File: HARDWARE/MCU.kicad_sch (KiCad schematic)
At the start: 1 part, among them U2 STM32H750VBTx

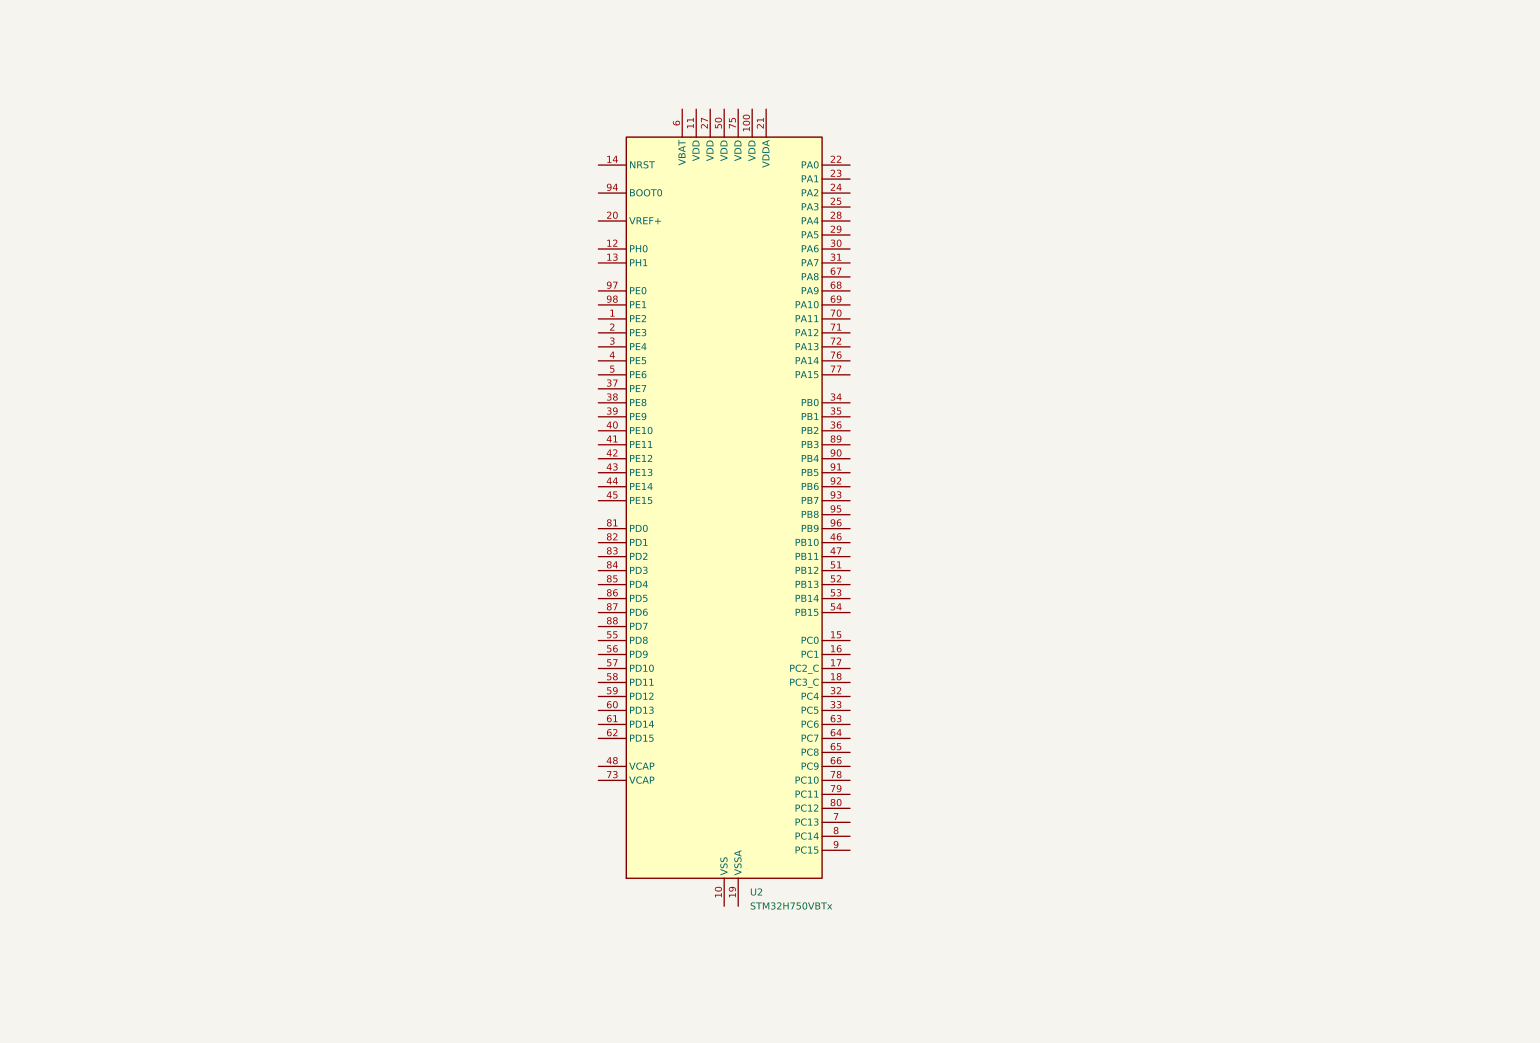
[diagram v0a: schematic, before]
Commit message: Update first version of schematic
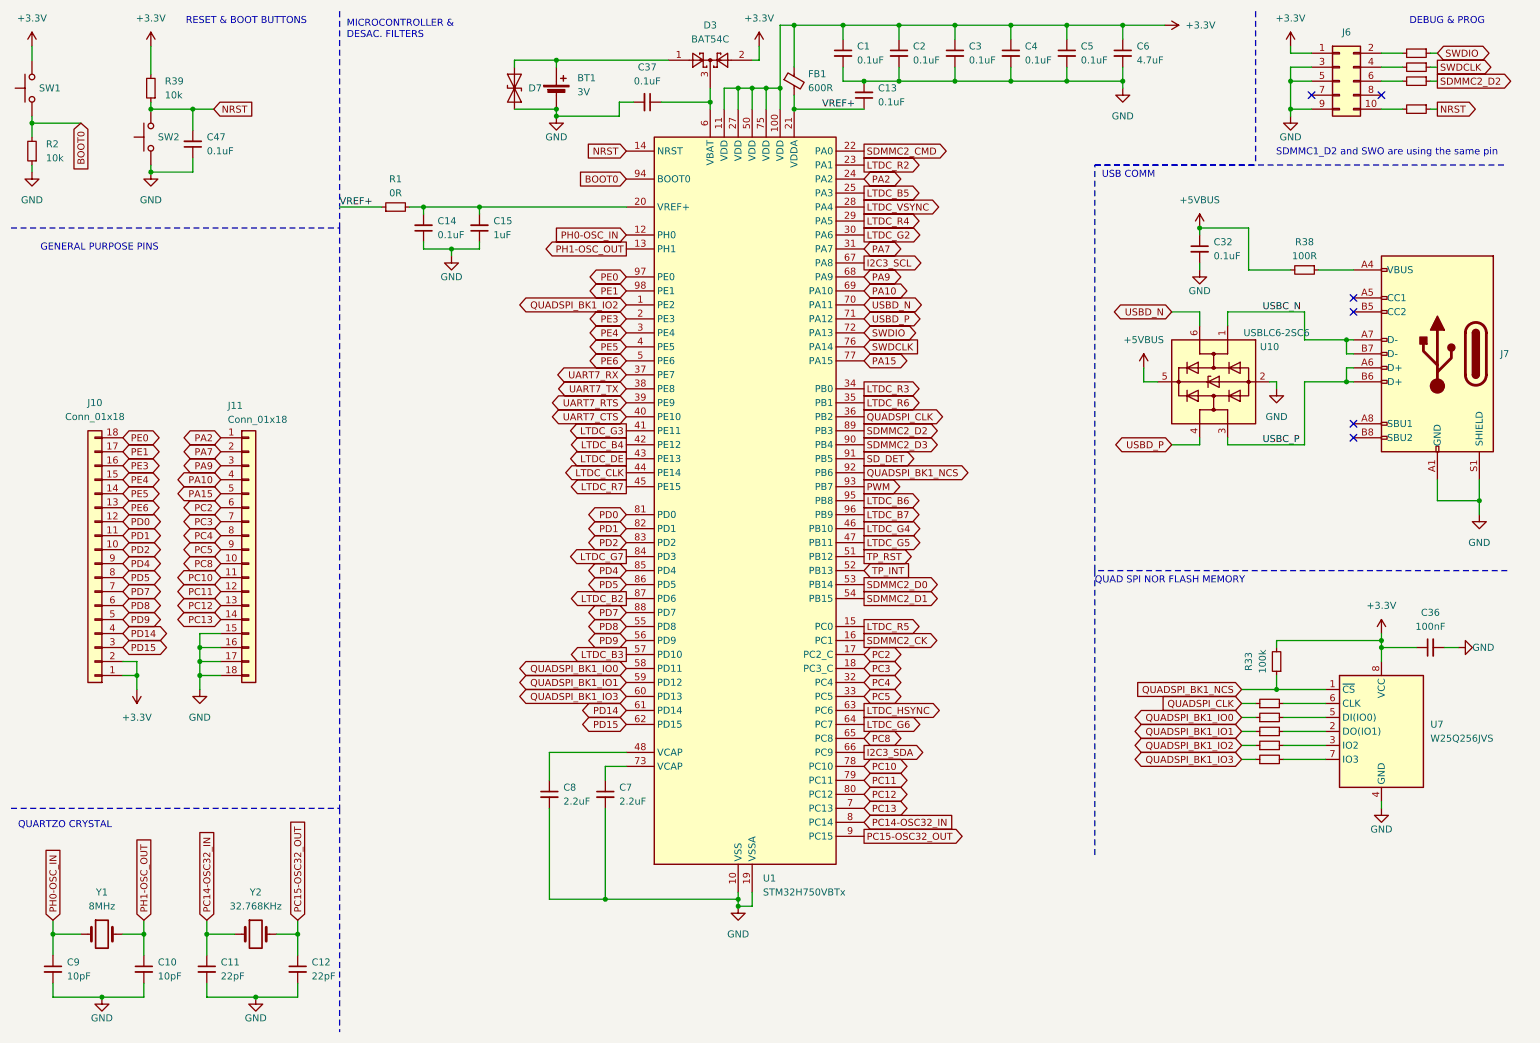
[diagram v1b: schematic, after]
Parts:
- removed U2: STM32H750VBTx, Package_QFP:LQFP-100_14x14mm_P0.5mm, symbol MCU_ST_STM32H7:STM32H750VBTx
- added BT1: 3V, BS-12-B-___002:BS-12-B-1A, symbol Device:Battery_Cell
- added C1, C13, C14, C2, C3, C32, C37, C4, C47, C5: 0.1uF, Capacitor_SMD:C_0603_1608Metric, symbol Device:C_Small
- added C10, C9: 10pF, Capacitor_SMD:C_0603_1608Metric, symbol Device:C_Small
- added C11, C12: 22pF, Capacitor_SMD:C_0603_1608Metric, symbol Device:C_Small
- added C15: 1uF, Capacitor_SMD:C_0603_1608Metric, symbol Device:C_Small
- added C36: 100nF, Capacitor_SMD:C_0603_1608Metric, symbol Device:C_Small
- added C6: 4.7uF, Capacitor_SMD:C_0603_1608Metric, symbol Device:C_Small
- added C7, C8: 2.2uF, Capacitor_SMD:C_0603_1608Metric, symbol Device:C_Small
- added D3: BAT54C, Package_TO_SOT_SMD:SOT-23, symbol Diode:BAT54C
- added D7: ESD9B3.3ST5G, Diode_SMD:D_SOD-923, symbol Diode:ESD9B3.3ST5G
- added FB1: 600R, Inductor_SMD:L_0603_1608Metric, symbol Device:FerriteBead_Small
- added J10, J11: Conn_01x18, Connector_JST:JST_XA_B18B-XASK-1_1x18_P2.50mm_Vertical, symbol Connector_Generic:Conn_01x18
- added J6: Conn_02x05_Odd_Even, Connector_PinHeader_1.27mm:PinHeader_2x05_P1.27mm_Vertical_SMD, symbol Connector_Generic:Conn_02x05_Odd_Even
- added J7: USB_C_Receptacle_USB2.0, Connector_USB:USB_C_Receptacle_G-Switch_GT-USB-7010ASV, symbol Connector:USB_C_Receptacle_USB2.0
- added R1: 0R, Resistor_SMD:R_0603_1608Metric, symbol Device:R_Small
- added R2, R39: 10k, Resistor_SMD:R_0603_1608Metric, symbol Device:R_Small
- added R28, R29, R30, R31, R32: 33R, Resistor_SMD:R_0603_1608Metric, symbol Device:R_Small
- added R33: 100k, Resistor_SMD:R_0603_1608Metric, symbol Device:R_Small
- added R34, R35, R36, R37: 22R, Resistor_SMD:R_0603_1608Metric, symbol Device:R_Small
- added R38: 100R, Resistor_SMD:R_0603_1608Metric, symbol Device:R_Small
- added SW1, SW2: SW_Push, Button_Switch_SMD:SW_SPST_CK_RS282G05A3, symbol Switch:SW_Push
- added U1: STM32H750VBTx, Package_QFP:LQFP-100_14x14mm_P0.5mm, symbol MCU_ST_STM32H7:STM32H750VBTx
- added U10: USBLC6-2SC6, Package_TO_SOT_SMD:SOT-23-6, symbol Power_Protection:USBLC6-2SC6
- added U7: W25Q256JVS, Package_SON:WSON-8-1EP_8x6mm_P1.27mm_EP3.4x4.3mm, symbol Memory_Flash:W25Q128JVS
- added Y1: 8MHz, Crystal:Crystal_SMD_Abracon_ABM3-2Pin_5.0x3.2mm, symbol Device:Crystal
- added Y2: 32.768KHz, Crystal:Crystal_SMD_3215-2Pin_3.2x1.5mm, symbol Device:Crystal
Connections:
- new net: R32.2, U7.6 (CLK)
- new net: J6.10 (Pin_10), R37.2
- new net: BT1.1 (+), D3.1, D7.2 (A2)
- new net: R31.2, U7.7 (IO3)
- new net: R29.2, U7.2 (DO(IO1))
- new net: R30.2, U7.3 (IO2)
- new net: R28.2, U7.5 (DI(IO0))
- new net: J6.2 (Pin_2), R34.2
- new net: C7.1, U1.73 (VCAP)
- new net: C14.2, C15.2, R1.2, U1.20 (VREF+)
- new net: J7.A4 (VBUS), J7.A9 (VBUS), J7.B4 (VBUS), J7.B9 (VBUS), R38.1
- new net: J6.4 (Pin_4), R35.2
- new net: J6.6 (Pin_6), R36.2
- new net: C8.1, U1.48 (VCAP)
- new net: C37.1, D3.3, U1.6 (VBAT)
- new net +3.3V: C1.1, C2.1, C3.1, C36.1, C4.1, C5.1, C6.1, D3.2, FB1.1, J10.1 (Pin_1), J10.2 (Pin_2), J6.1 (Pin_1), R33.2, R39.2, SW1.2, U1.100 (VDD), U1.11 (VDD), U1.27 (VDD), U1.50 (VDD), U1.75 (VDD), U7.8 (VCC)
- new net +5VBUS: C32.1, R38.2, U10.5 (VBUS)
- new net BOOT0: R2.2, SW1.1, U1.94 (BOOT0)
- new net GND: BT1.2 (-), C1.2, C10.2, C11.2, C12.2, C13.2, C14.1, C15.1, C2.2, C3.2, C32.2, C36.2, C37.2, C4.2, C47.1, C5.2, C6.2, C7.2, C8.2, C9.2, D7.1 (A1), J11.15 (Pin_15), J11.16 (Pin_16), J11.17 (Pin_17), J11.18 (Pin_18), J6.3 (Pin_3), J6.5 (Pin_5), J6.9 (Pin_9), J7.A1 (GND), J7.A12 (GND), J7.B1 (GND), J7.B12 (GND), J7.S1 (SHIELD), R2.1, SW2.1, U1.10 (VSS), U1.19 (VSSA), U1.26 (VSS), U1.49 (VSS), U1.74 (VSS), U1.99 (VSS), U10.2 (GND), U7.4 (GND)
- new net I2C3_SCL: U1.67 (PA8)
- new net I2C3_SDA: U1.66 (PC9)
- new net LTDC_B2: U1.87 (PD6)
- new net LTDC_B3: U1.57 (PD10)
- new net LTDC_B4: U1.42 (PE12)
- new net LTDC_B5: U1.25 (PA3)
- new net LTDC_B6: U1.95 (PB8)
- new net LTDC_B7: U1.96 (PB9)
- new net LTDC_CLK: U1.44 (PE14)
- new net LTDC_DE: U1.43 (PE13)
- new net LTDC_G2: U1.30 (PA6)
- new net LTDC_G3: U1.41 (PE11)
- new net LTDC_G4: U1.46 (PB10)
- new net LTDC_G5: U1.47 (PB11)
- new net LTDC_G6: U1.64 (PC7)
- new net LTDC_G7: U1.84 (PD3)
- new net LTDC_HSYNC: U1.63 (PC6)
- new net LTDC_R2: U1.23 (PA1)
- new net LTDC_R3: U1.34 (PB0)
- new net LTDC_R4: U1.29 (PA5)
- new net LTDC_R5: U1.15 (PC0)
- new net LTDC_R6: U1.35 (PB1)
- new net LTDC_R7: U1.45 (PE15)
- new net LTDC_VSYNC: U1.28 (PA4)
- new net NRST: C47.2, R37.1, R39.1, SW2.2, U1.14 (NRST)
- new net PA10: J11.4 (Pin_4), U1.69 (PA10)
- new net PA15: J11.5 (Pin_5), U1.77 (PA15)
- new net PA2: J11.1 (Pin_1), U1.24 (PA2)
- new net PA7: J11.2 (Pin_2), U1.31 (PA7)
- new net PA9: J11.3 (Pin_3), U1.68 (PA9)
- new net PC10: J11.11 (Pin_11), U1.78 (PC10)
- new net PC11: J11.12 (Pin_12), U1.79 (PC11)
- new net PC12: J11.13 (Pin_13), U1.80 (PC12)
- new net PC13: J11.14 (Pin_14), U1.7 (PC13)
- new net PC14-OSC32_IN: C11.1, U1.8 (PC14), Y2.1
- new net PC15-OSC32_OUT: C12.1, U1.9 (PC15), Y2.2
- new net PC2: J11.6 (Pin_6), U1.17 (PC2_C)
- new net PC3: J11.7 (Pin_7), U1.18 (PC3_C)
- new net PC4: J11.8 (Pin_8), U1.32 (PC4)
- new net PC5: J11.9 (Pin_9), U1.33 (PC5)
- new net PC8: J11.10 (Pin_10), U1.65 (PC8)
- new net PD0: J10.12 (Pin_12), U1.81 (PD0)
- new net PD1: J10.11 (Pin_11), U1.82 (PD1)
- new net PD14: J10.4 (Pin_4), U1.61 (PD14)
- new net PD15: J10.3 (Pin_3), U1.62 (PD15)
- new net PD2: J10.10 (Pin_10), U1.83 (PD2)
- new net PD4: J10.9 (Pin_9), U1.85 (PD4)
- new net PD5: J10.8 (Pin_8), U1.86 (PD5)
- new net PD7: J10.7 (Pin_7), U1.88 (PD7)
- new net PD8: J10.6 (Pin_6), U1.55 (PD8)
- new net PD9: J10.5 (Pin_5), U1.56 (PD9)
- new net PE0: J10.18 (Pin_18), U1.97 (PE0)
- new net PE1: J10.17 (Pin_17), U1.98 (PE1)
- new net PE3: J10.16 (Pin_16), U1.2 (PE3)
- new net PE4: J10.15 (Pin_15), U1.3 (PE4)
- new net PE5: J10.14 (Pin_14), U1.4 (PE5)
- new net PE6: J10.13 (Pin_13), U1.5 (PE6)
- new net PH0-OSC_IN: C9.1, U1.12 (PH0), Y1.1
- new net PH1-OSC_OUT: C10.1, U1.13 (PH1), Y1.2
- new net PWM: U1.93 (PB7)
- new net QUADSPI_BK1_IO0: R28.1, U1.58 (PD11)
- new net QUADSPI_BK1_IO1: R29.1, U1.59 (PD12)
- new net QUADSPI_BK1_IO2: R30.1, U1.1 (PE2)
- new net QUADSPI_BK1_IO3: R31.1, U1.60 (PD13)
- new net QUADSPI_BK1_NCS: R33.1, U1.92 (PB6), U7.1 (~{CS})
- new net QUADSPI_CLK: R32.1, U1.36 (PB2)
- new net SDMMC2_CK: U1.16 (PC1)
- new net SDMMC2_CMD: U1.22 (PA0)
- new net SDMMC2_D0: U1.53 (PB14)
- new net SDMMC2_D1: U1.54 (PB15)
- new net SDMMC2_D2: R36.1, U1.89 (PB3)
- new net SDMMC2_D3: U1.90 (PB4)
- new net SD_DET: U1.91 (PB5)
- new net SWDCLK: R35.1, U1.76 (PA14)
- new net SWDIO: R34.1, U1.72 (PA13)
- new net TP_INT: U1.52 (PB13)
- new net TP_RST: U1.51 (PB12)
- new net UART7_CTS: U1.40 (PE10)
- new net UART7_RTS: U1.39 (PE9)
- new net UART7_RX: U1.37 (PE7)
- new net UART7_TX: U1.38 (PE8)
- new net USBC_N: J7.A7 (D-), J7.B7 (D-), U10.1 (I/O1)
- new net USBC_P: J7.A6 (D+), J7.B6 (D+), U10.3 (I/O2)
- new net USBD_N: U1.70 (PA11), U10.6 (I/O1)
- new net USBD_P: U1.71 (PA12), U10.4 (I/O2)
- new net VREF+: C13.1, FB1.2, R1.1, U1.21 (VDDA)
- no-connect marks 0 -> 6
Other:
- note added: "DEBUG & PROG"
- note added: "GENERAL PURPOSE PINS"
- note added: "MICROCONTROLLER & DESAC. FILTERS"
- note added: "QUAD SPI NOR FLASH MEMORY"
- note added: "QUARTZO CRYSTAL"
- note added: "RESET & BOOT BUTTONS"
- note added: "SDMMC1_D2 and SWO are using the same pin"
- note added: "USB COMM"
